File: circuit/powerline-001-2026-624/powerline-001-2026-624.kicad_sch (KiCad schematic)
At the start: 10 parts, among them J1 Conn_01x03_Pin, J10 Conn_01x02_Pin, J2 Conn_02x05_Odd_Even, J3 Conn_02x08_Odd_Even, J4 Conn_02x09_Odd_Even, J5 Conn_01x02_Pin, J6 Conn_01x02_Pin, J7 Conn_01x02_Pin, J8 Conn_01x02_Pin, J9 Conn_01x02_Pin

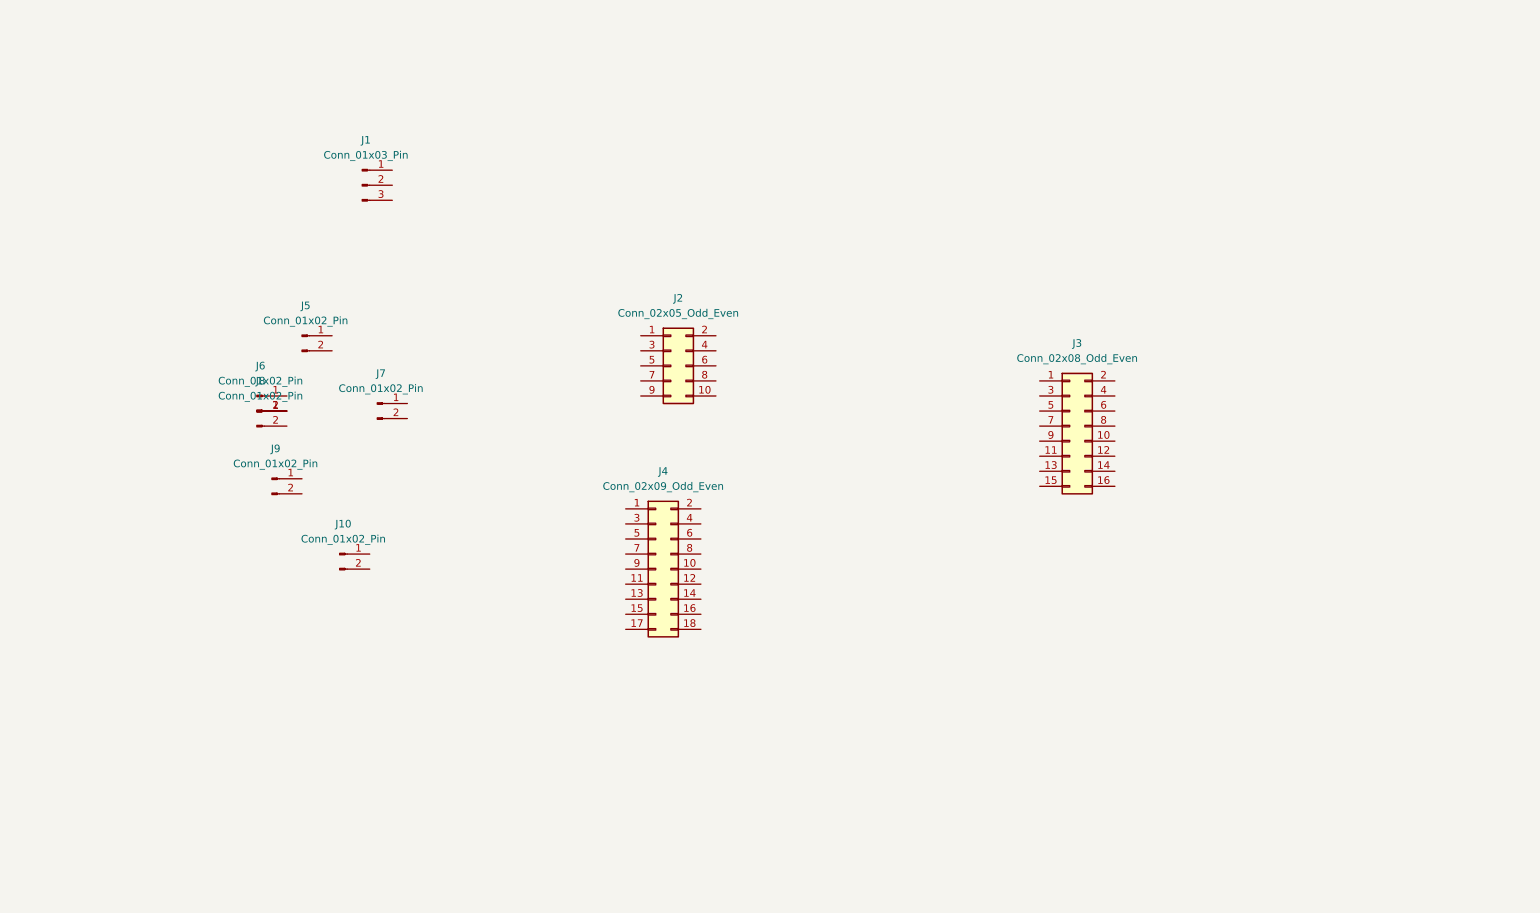
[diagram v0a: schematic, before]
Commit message: Create 供給基板の回路図完成
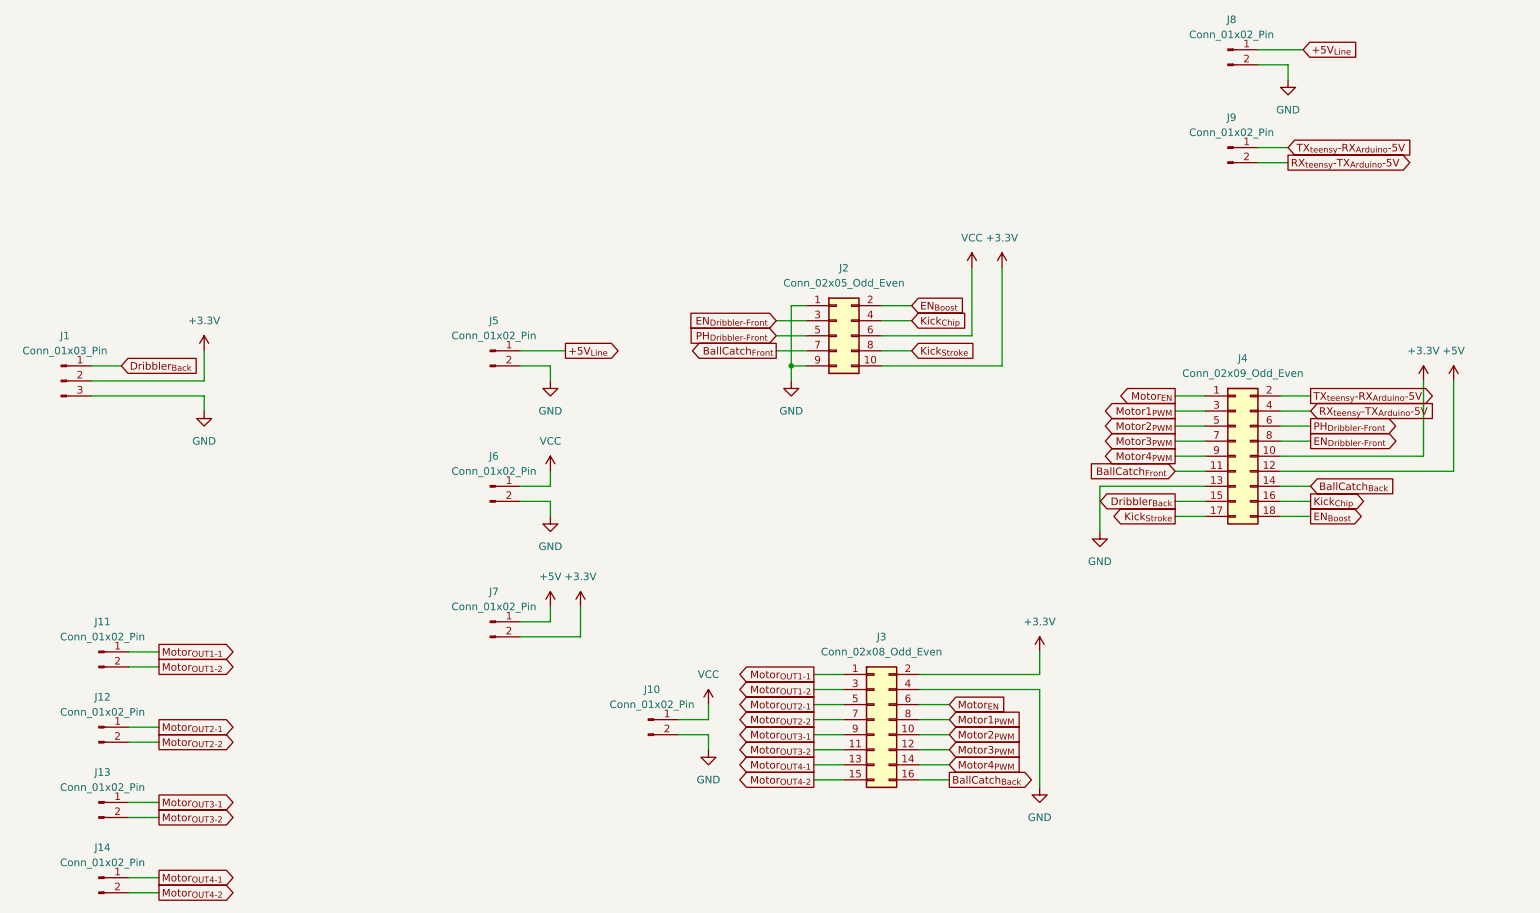
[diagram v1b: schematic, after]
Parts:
- added J11, J12, J13, J14: Conn_01x02_Pin, symbol Connector:Conn_01x02_Pin
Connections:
- net GND: now reaches J2.1 (Pin_1)
- net GND: now also J1.3 (Pin_3), J10.2 (Pin_2), J2.9 (Pin_9), J3.4 (Pin_4), J4.13 (Pin_13), J5.2 (Pin_2), J6.2 (Pin_2), J8.2 (Pin_2)
- net +3.3V: now reaches J2.10 (Pin_10)
- net +3.3V: now also J1.2 (Pin_2), J3.2 (Pin_2), J4.10 (Pin_10), J7.2 (Pin_2)
- net EN_{Boost}: now reaches J2.2 (Pin_2)
- net EN_{Boost}: now also J4.18 (Pin_18)
- net EN_{Dribbler-Front}: now reaches J2.3 (Pin_3)
- net EN_{Dribbler-Front}: now also J4.8 (Pin_8)
- net Kick_{Chip}: now reaches J2.4 (Pin_4)
- net Kick_{Chip}: now also J4.16 (Pin_16)
- net PH_{Dribbler-Front}: now reaches J2.5 (Pin_5)
- net PH_{Dribbler-Front}: now also J4.6 (Pin_6)
- net VCC: now reaches J2.6 (Pin_6)
- net VCC: now also J10.1 (Pin_1), J6.1 (Pin_1)
- net BallCatch_{Front}: now reaches J2.7 (Pin_7)
- net BallCatch_{Front}: now also J4.11 (Pin_11)
- net Kick_{Stroke}: now reaches J2.8 (Pin_8)
- net Kick_{Stroke}: now also J4.17 (Pin_17)
- net +5V_{Line}: now reaches J8.1 (Pin_1)
- net +5V_{Line}: now also J5.1 (Pin_1); no longer J6.2 (Pin_2)
- net Motor_{OUT1-1}: now reaches J3.1 (Pin_1)
- net Motor_{OUT1-1}: now also J11.1 (Pin_1)
- net Motor2_{PWM}: now reaches J3.10 (Pin_10)
- net Motor2_{PWM}: now also J4.5 (Pin_5)
- net Motor_{OUT3-2}: now reaches J3.11 (Pin_11)
- net Motor_{OUT3-2}: now also J13.2 (Pin_2)
- net Motor3_{PWM}: now reaches J3.12 (Pin_12)
- net Motor3_{PWM}: now also J4.7 (Pin_7)
- net Motor_{OUT4-1}: now reaches J3.13 (Pin_13)
- net Motor_{OUT4-1}: now also J14.1 (Pin_1)
- net Motor4_{PWM}: now reaches J3.14 (Pin_14)
- net Motor4_{PWM}: now also J4.9 (Pin_9)
- net Motor_{OUT4-2}: now reaches J3.15 (Pin_15)
- net Motor_{OUT4-2}: now also J14.2 (Pin_2)
- net BallCatch_{Back}: now reaches J3.16 (Pin_16)
- net BallCatch_{Back}: now also J4.14 (Pin_14)
- net Motor_{OUT1-2}: now reaches J3.3 (Pin_3)
- net Motor_{OUT1-2}: now also J11.2 (Pin_2)
- net Motor_{OUT2-1}: now reaches J3.5 (Pin_5)
- net Motor_{OUT2-1}: now also J12.1 (Pin_1)
- net Motor_{EN}: now reaches J3.6 (Pin_6)
- net Motor_{EN}: now also J4.1 (Pin_1)
- net Motor_{OUT2-2}: now reaches J3.7 (Pin_7)
- net Motor_{OUT2-2}: now also J12.2 (Pin_2)
- net Motor1_{PWM}: now reaches J3.8 (Pin_8)
- net Motor1_{PWM}: now also J4.3 (Pin_3)
- net Motor_{OUT3-1}: now reaches J3.9 (Pin_9)
- net Motor_{OUT3-1}: now also J13.1 (Pin_1)
- net +5V: now reaches J4.12 (Pin_12)
- net +5V: now also J7.1 (Pin_1)
- net Dribbler_{Back}: now reaches J4.15 (Pin_15)
- net Dribbler_{Back}: now also J1.1 (Pin_1)
- net TX_{teensy}-RX_{Arduino}-5V: now reaches J4.2 (Pin_2)
- net TX_{teensy}-RX_{Arduino}-5V: now also J9.1 (Pin_1)
- net RX_{teensy}-TX_{Arduino}-5V: now reaches J4.4 (Pin_4)
- net RX_{teensy}-TX_{Arduino}-5V: now also J9.2 (Pin_2)
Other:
- moved on the sheet: J1, J2, J3, J4, J5
